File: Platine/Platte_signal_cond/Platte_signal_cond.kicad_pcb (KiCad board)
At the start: 2 copper layers, 28 parts, among them J1 Conn_01x06, J2 Conn_01x07_MountingPin

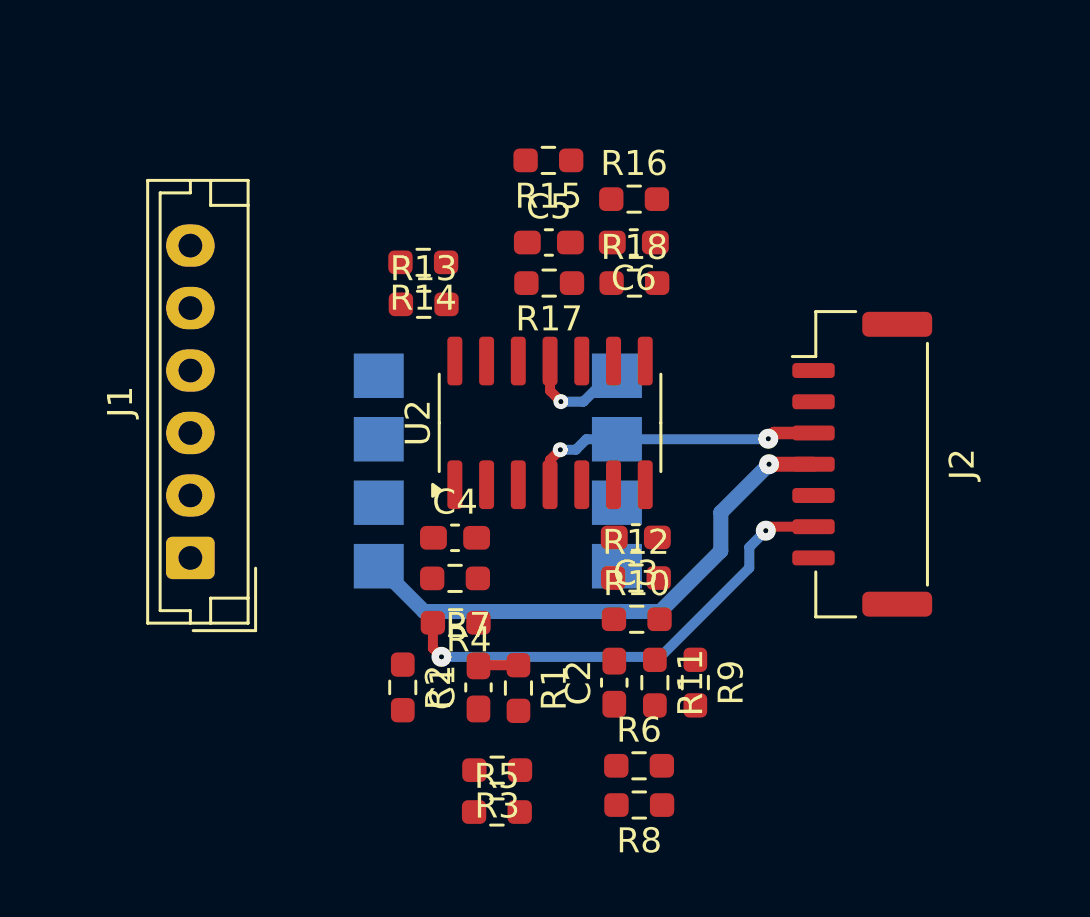
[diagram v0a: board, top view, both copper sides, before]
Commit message: Both the PCBs finished
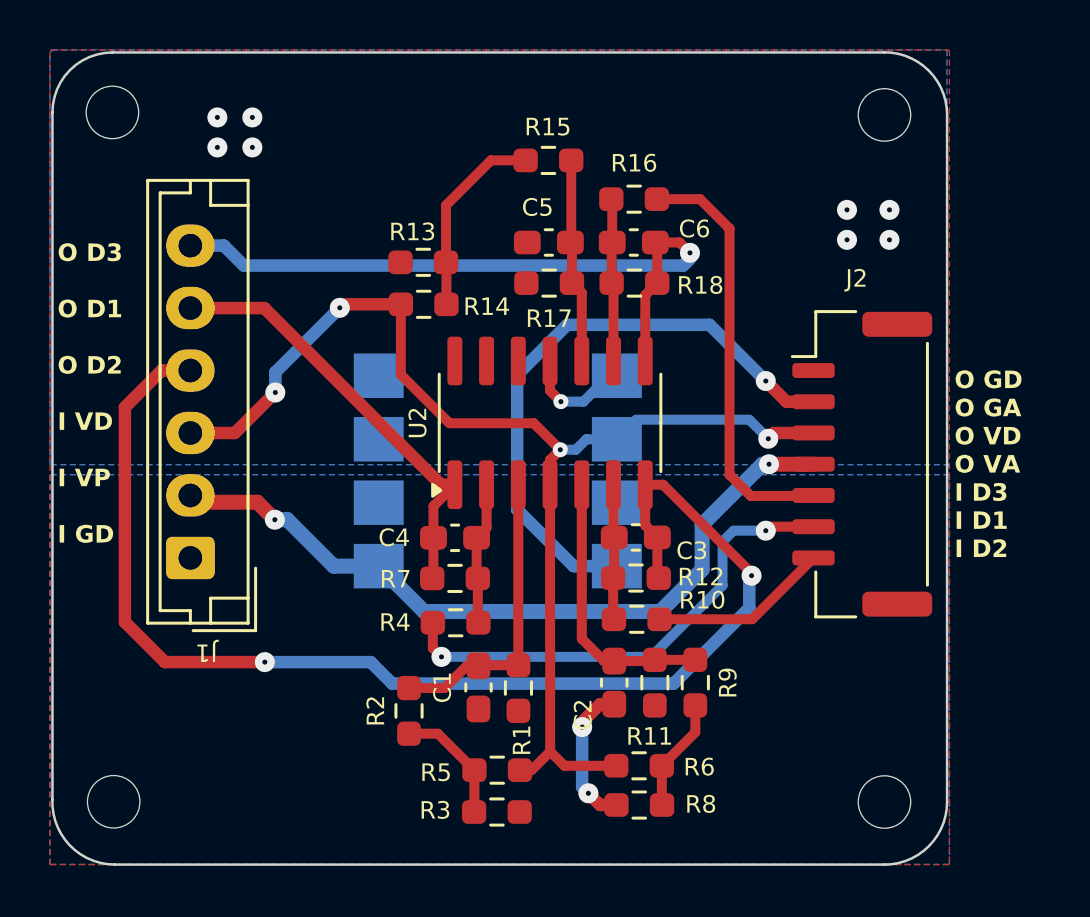
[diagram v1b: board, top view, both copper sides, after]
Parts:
- added M1: MountingHole_2.1mm, MountingHole:MountingHole_2.1mm, F.Cu at (93.6, 62.2)
- added M2: MountingHole_2.1mm, MountingHole:MountingHole_2.1mm, F.Cu at (124.5, 62.3)
- added M3: MountingHole_2.1mm, MountingHole:MountingHole_2.1mm, F.Cu at (93.7, 89.8)
- added M4: MountingHole_2.1mm, MountingHole:MountingHole_2.1mm, F.Cu at (124.5, 89.8)
- moved R2 0.97 mm to (105.5, 86.2)
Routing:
- net /Out2: track 0.00 -> 50.2 mm, vias 0 -> 2
- net +3.3VD: track 12.0 -> 49.2 mm, vias 2 -> 4
- net /Out3: track 0.00 -> 27.2 mm, vias 0 -> 1
- net GNDA: track 0.00 -> 24.3 mm, vias 0 -> 1
- net /Out1: track 0.00 -> 17.6 mm
- net /data_in3: track 0.00 -> 17.0 mm
- net /Vin2+: track 0.00 -> 11.1 mm
- net /Vin1+: track 1.61 -> 12.0 mm
- net +3.3VA: track 21.5 -> 30.4 mm, vias 1 -> 2
- net /Vin3+: track 0.00 -> 8.23 mm
- net Net-(R13-Pad2): track 0.00 -> 7.90 mm
- net /data_in2: track 0.00 -> 7.18 mm
- net /Vin3-: track 0.00 -> 6.54 mm
- net GNDD: track 4.47 -> 10.3 mm, vias 1 -> 11
- net /Vin1-: track 0.00 -> 5.72 mm
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- added copper zone on B.Cu, net GNDA
- added copper zone on B.Cu, net GNDD
- added copper zone on F.Cu, net GNDD
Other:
- board outline added: 35.8 x 32.5 mm
- board text added: "O D3 O D1 O D2 I VD I VP I GD"
- board text added: "O GD O GA O VD O VA I D3 I D1 I D2"
